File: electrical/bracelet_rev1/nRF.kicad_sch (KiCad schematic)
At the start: 26 parts, among them J2 Conn_01x04_Pin, SW1 SW_Push, U1 nRF54L10-QFXX, Y1 Crystal_GND24

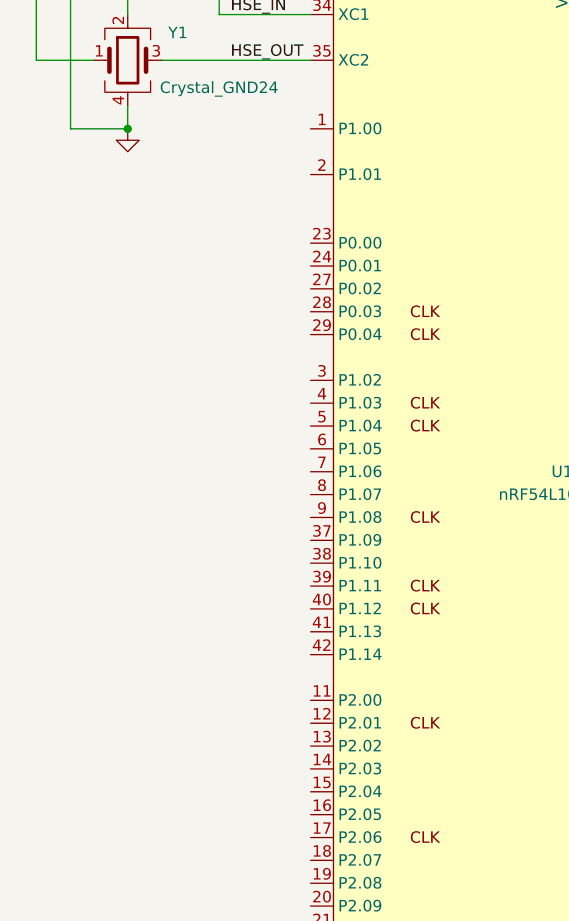
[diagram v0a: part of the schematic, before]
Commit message: Mostly finihsed hopefully but still needs clean up anyway
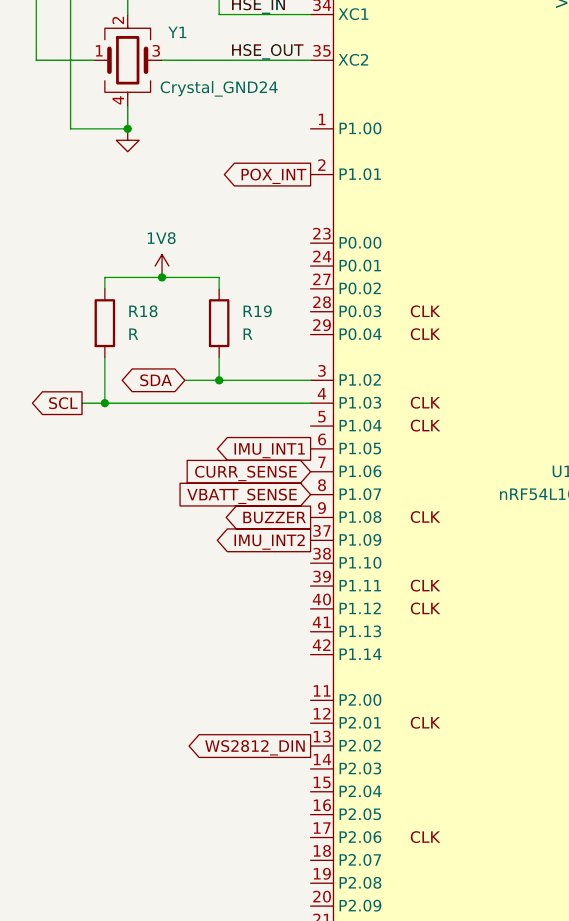
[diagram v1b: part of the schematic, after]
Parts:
- added R18, R19: R, symbol Device:R
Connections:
- net 1V8: now also R18.1, R19.1
- net WS2812_DIN: now reaches U1.13 (P2.02)
- net POX_INT: now reaches U1.2 (P1.01)
- net SDA: now reaches U1.3 (P1.02)
- net SDA: now also R19.2
- net IMU_INT2: now reaches U1.37 (P1.09)
- net SCL: now reaches U1.4 (P1.03)
- net SCL: now also R18.2
- net IMU_INT1: now reaches U1.6 (P1.05)
- net CURR_SENSE: now reaches U1.7 (P1.06)
- net VBATT_SENSE: now reaches U1.8 (P1.07)
- net BUZZER: now reaches U1.9 (P1.08)
